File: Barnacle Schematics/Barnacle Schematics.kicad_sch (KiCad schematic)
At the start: 17 parts, among them M3 MG996, M4 SG90, SW1 Reset, U1 TiVa

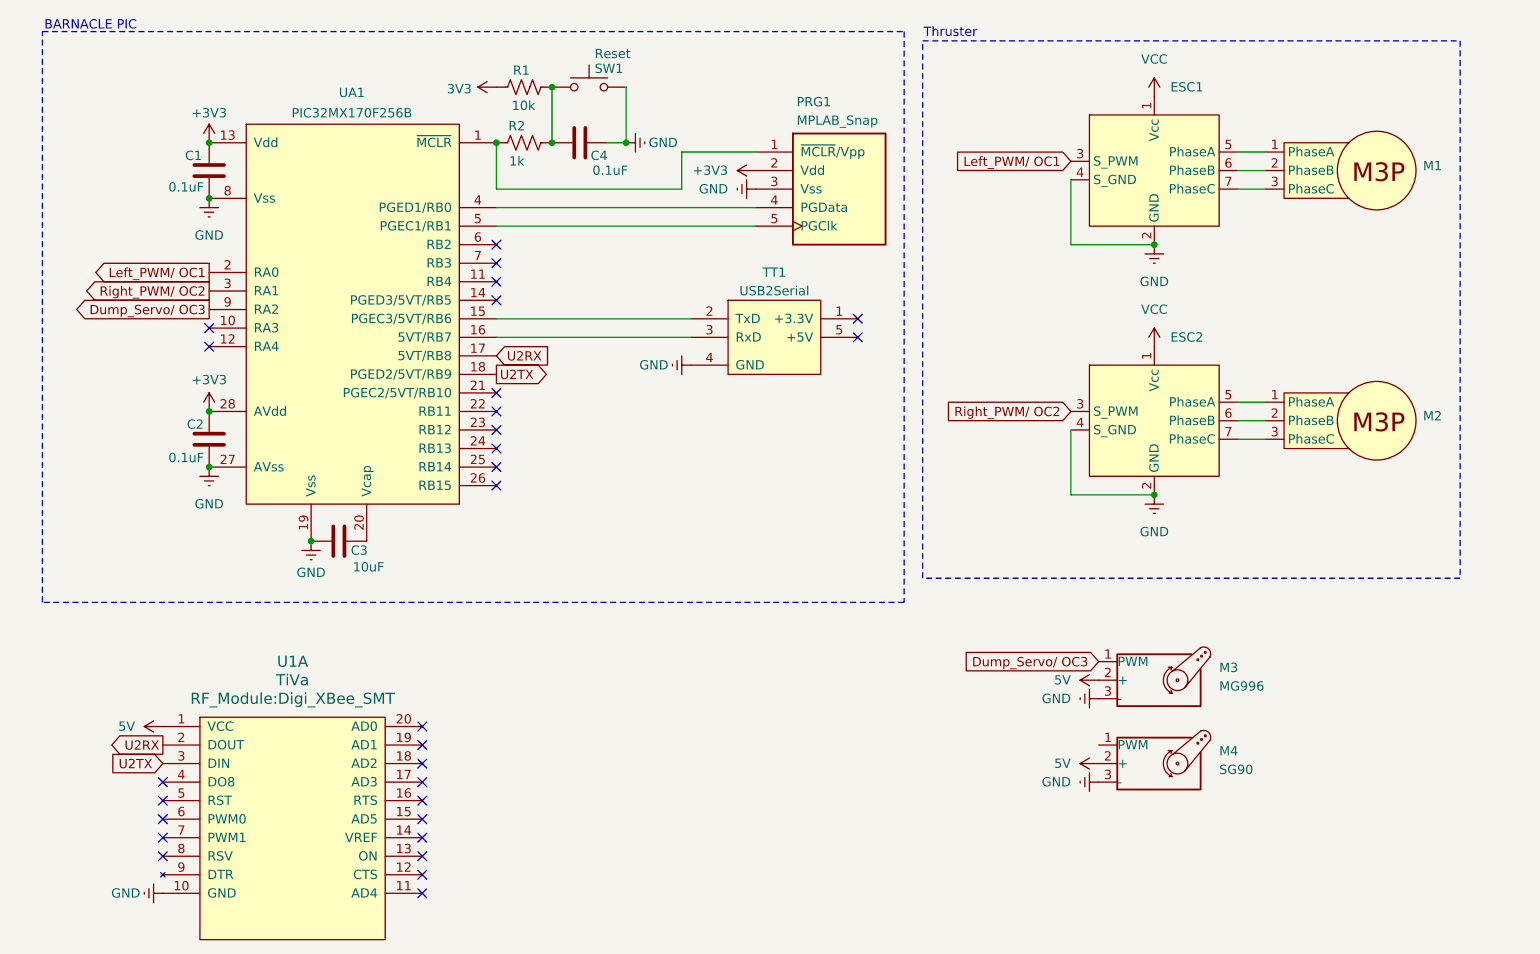
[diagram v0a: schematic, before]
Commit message: power global bariable and some other update
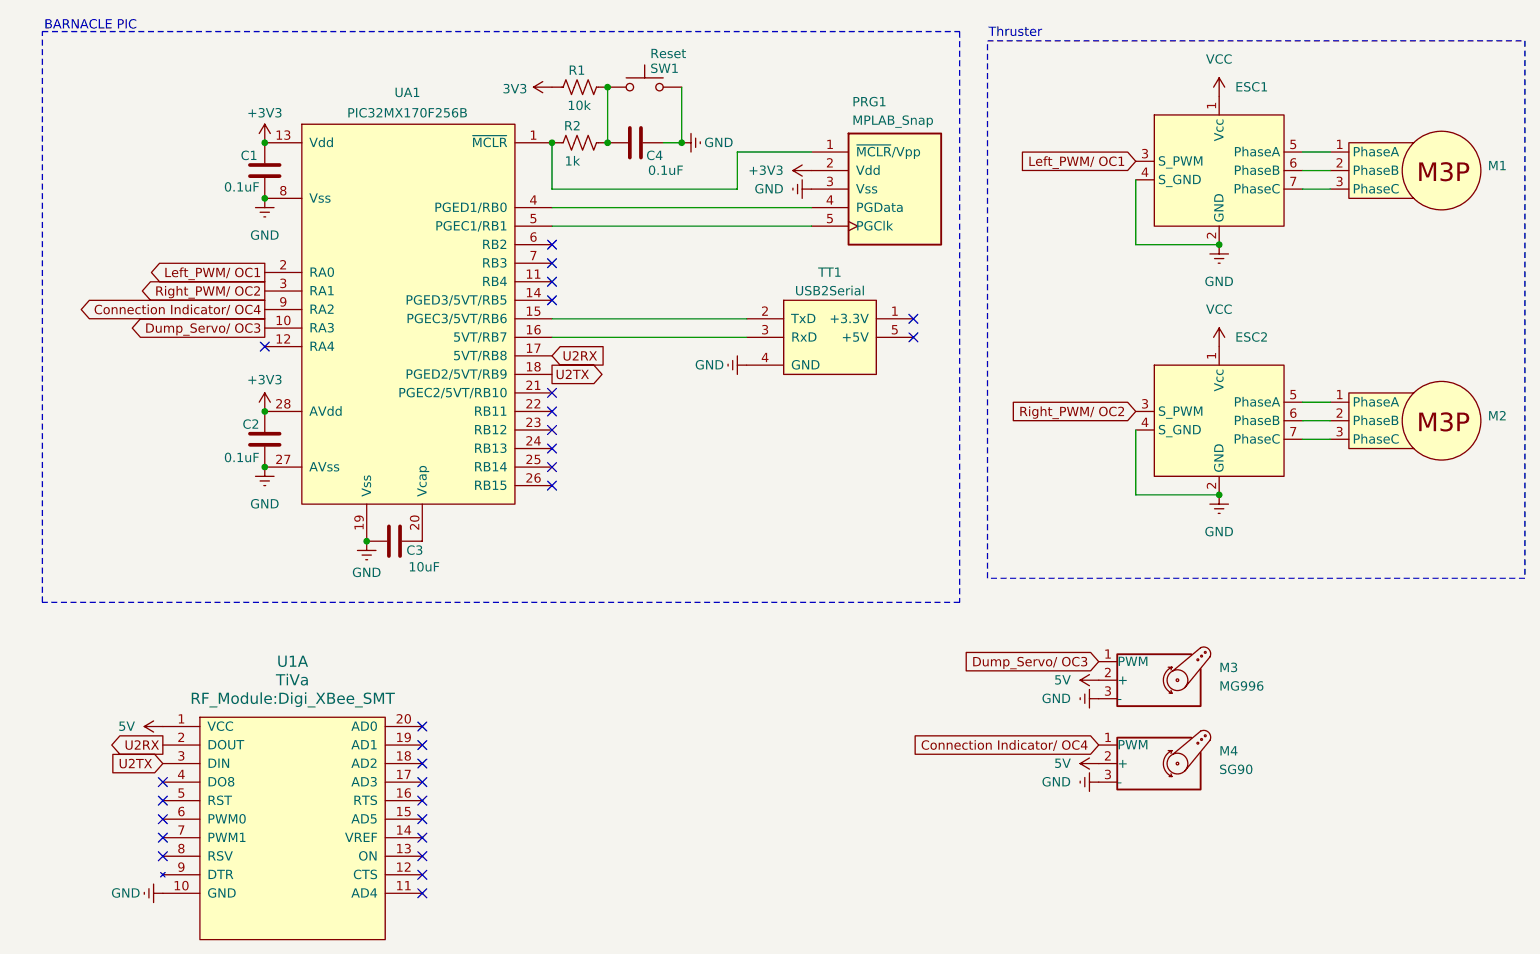
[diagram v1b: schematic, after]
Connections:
- net Dump_Servo/ OC3: now also UA1.10 (RA3); no longer UA1.9 (RA2)
- net Connection Indicator/ OC4: now reaches M4.1 (PWM)
- net Connection Indicator/ OC4: now also UA1.9 (RA2)
- no-connect marks 29 -> 28
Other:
- moved on the sheet: C1, C2, C3, C4, ESC1, ESC2, M1, M2, PRG1, R1, R2, SW1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
